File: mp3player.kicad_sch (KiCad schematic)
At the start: 6 parts, among them J1 AudioJack3, U1 ES8388, U2 ESP32-S3-WROOM-1

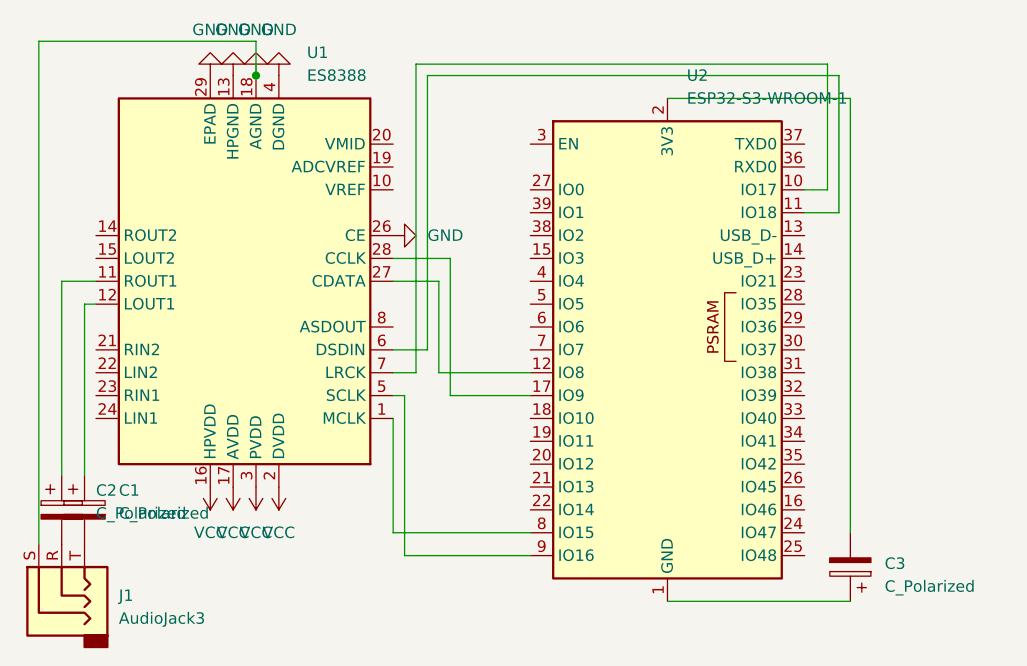
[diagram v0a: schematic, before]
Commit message: Autosave
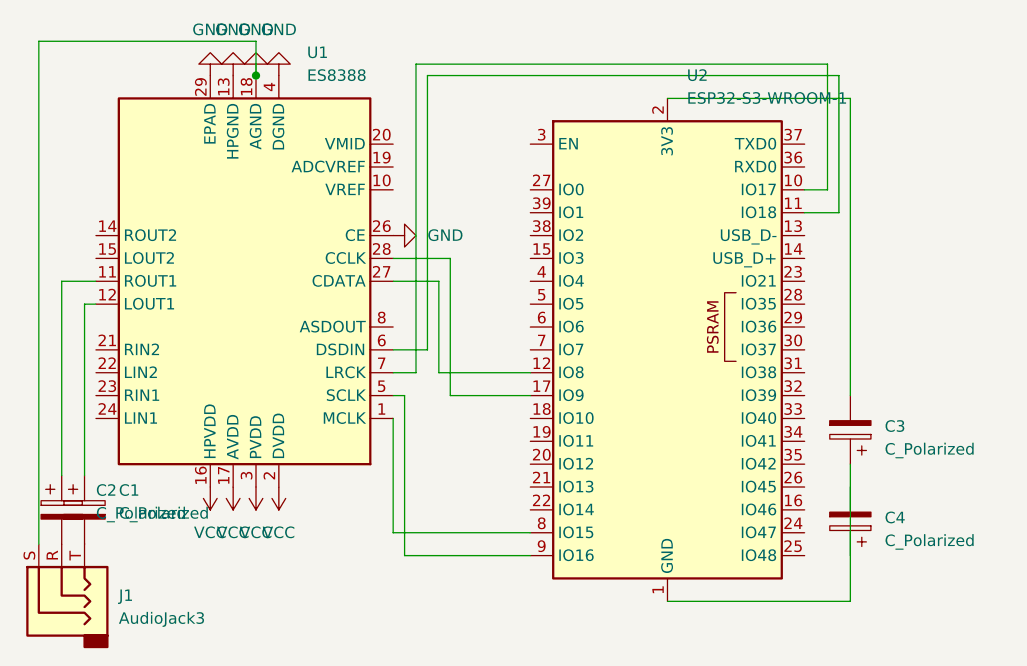
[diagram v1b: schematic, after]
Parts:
- added C4: C_Polarized, symbol Device:C_Polarized
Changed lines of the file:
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@@
 	(wire
 		(pts
-			(xy 105.41 19.05) (xy 105.41 67.31)
+			(xy 105.41 19.05) (xy 105.41 52.07)
 		)
 		(stroke
@@
 	(wire
 		(pts
-			(xy 21.59 41.91) (xy 20.32 41.91)
+			(xy 105.41 59.69) (xy 105.41 74.93)
 		)
 		(stroke
@@
 	(wire
 		(pts
-			(xy 59.69 49.53) (xy 69.85 49.53)
+			(xy 21.59 41.91) (xy 20.32 41.91)
 		)
 		(stroke
@@
 	(wire
 		(pts
-			(xy 58.42 46.99) (xy 54.61 46.99)
+			(xy 59.69 49.53) (xy 69.85 49.53)
 		)
 		(stroke
@@
 	(wire
 		(pts
-			(xy 58.42 16.51) (xy 58.42 46.99)
+			(xy 58.42 46.99) (xy 54.61 46.99)
 		)
 		(stroke
@@
 		)
 	)
+	(wire
+		(pts
+			(xy 58.42 16.51) (xy 58.42 46.99)
+		)
+		(stroke
+			(width 0)
+			(type default)
+		)
+	)
 	(symbol
 		(lib_id "power:VCC")
@@
 	)
 	(symbol
+		(lib_id "Device:C_Polarized")
+		(at 105.41 66.04 180)
+		(unit 1)
+		(body_style 1)
+		(exclude_from_sim no)
+		(in_bom yes)
+		(on_board yes)
+		(in_pos_files yes)
+		(dnp no)
+		(fields_autoplaced yes)
+		(property "Reference" "C4"
+			(at 109.22 65.6589 0)
+			(show_name no)
+			(do_not_autoplace no)
+			(effects
+				(font
+					(size 1.27 1.27)
+				)
+				(justify right)
+			)
+		)
+		(property "Value" "C_Polarized"
+			(at 109.22 68.1989 0)
+			(show_name no)
+			(do_not_autoplace no)
+			(effects
+				(font
+					(size 1.27 1.27)
+				)
+				(justify right)
+			)
+		)
+		(property "Footprint" ""
+			(at 104.4448 62.23 0)
+			(hide yes)
+			(show_name no)
+			(do_not_autoplace no)
+			(effects
+				(font
+					(size 1.27 1.27)
+				)
+			)
+		)
+		(property "Datasheet" ""
+			(at 105.41 66.04 0)
+			(hide yes)
+			(show_name no)
+			(do_not_autoplace no)
+			(effects
+				(font
+					(size 1.27 1.27)
+				)
+			)
+		)
+		(property "Description" "Polarized capacitor"
+			(at 105.41 66.04 0)
+			(hide yes)
+			(show_name no)
+			(do_not_autoplace no)
+			(effects
+				(font
+					(size 1.27 1.27)
+				)
+			)
+		)
+		(pin "1"
+		)
+		(pin "2"
+		)
+		(instances
+			(project "mp3player"
+				(path "/7851373b-cb7e-4e42-801a-d8b5ac5735f4"
+					(reference "C4")
+					(unit 1)
+				)
+			)
+		)
+	)
+	(symbol
+		(lib_id "Device:C_Polarized")
+		(at 105.41 55.88 180)
+		(unit 1)
+		(body_style 1)
+		(exclude_from_sim no)
+		(in_bom yes)
+		(on_board yes)
+		(in_pos_files yes)
+		(dnp no)
+		(fields_autoplaced yes)
+		(property "Reference" "C3"
+			(at 109.22 55.4989 0)
+			(show_name no)
+			(do_not_autoplace no)
+			(effects
+				(font
+					(size 1.27 1.27)
+				)
+				(justify right)
+			)
+		)
+		(property "Value" "C_Polarized"
+			(at 109.22 58.0389 0)
+			(show_name no)
+			(do_not_autoplace no)
+			(effects
+				(font
+					(size 1.27 1.27)
+				)
+				(justify right)
+			)
+		)
+		(property "Footprint" ""
+			(at 104.4448 52.07 0)
+			(hide yes)
+			(show_name no)
+			(do_not_autoplace no)
+			(effects
+				(font
+					(size 1.27 1.27)
+				)
+			)
+		)
+		(property "Datasheet" ""
+			(at 105.41 55.88 0)
+			(hide yes)
+			(show_name no)
+			(do_not_autoplace no)
+			(effects
+				(font
+					(size 1.27 1.27)
+				)
+			)
+		)
+		(property "Description" "Polarized capacitor"
+			(at 105.41 55.88 0)
+			(hide yes)
+			(show_name no)
+			(do_not_autoplace no)
+			(effects
+				(font
+					(size 1.27 1.27)
+				)
+			)
+		)
+		(pin "1"
+		)
+		(pin "2"
+		)
+		(instances
+			(project "mp3player"
+				(path "/7851373b-cb7e-4e42-801a-d8b5ac5735f4"
+					(reference "C3")
+					(unit 1)
+				)
+			)
+		)
+	)
+	(symbol
 		(lib_id "Connector_Audio:AudioJack3")
 		(at 17.78 73.66 90)
@@
 					(unit 1)
 				)
-			)
-		)
-	)
-	(symbol
-		(lib_id "Device:C_Polarized")
-		(at 105.41 71.12 180)
-		(unit 1)
-		(body_style 1)
-		(exclude_from_sim no)
-		(in_bom yes)
-		(on_board yes)
-		(in_pos_files yes)
-		(dnp no)
-		(fields_autoplaced yes)
-		(property "Reference" "C3"
-			(at 109.22 70.7389 0)
-			(show_name no)
-			(do_not_autoplace no)
-			(effects
-				(font
-					(size 1.27 1.27)
-				)
-				(justify right)
-			)
-		)
-		(property "Value" "C_Polarized"
-			(at 109.22 73.2789 0)
-			(show_name no)
-			(do_not_autoplace no)
-			(effects
-				(font
-					(size 1.27 1.27)
-				)
-				(justify right)
-			)
-		)
-		(property "Footprint" ""
-			(at 104.4448 67.31 0)
-			(hide yes)
-			(show_name no)
-			(do_not_autoplace no)
-			(effects
-				(font
-					(size 1.27 1.27)
-				)
-			)
-		)
-		(property "Datasheet" ""
-			(at 105.41 71.12 0)
-			(hide yes)
-			(show_name no)
-			(do_not_autoplace no)
-			(effects
-				(font
-					(size 1.27 1.27)
-				)
-			)
-		)
-		(property "Description" "Polarized capacitor"
-			(at 105.41 71.12 0)
-			(hide yes)
-			(show_name no)
-			(do_not_autoplace no)
-			(effects
-				(font
-					(size 1.27 1.27)
-				)
-			)
-		)
-		(pin "1"
-		)
-		(pin "2"
-		)
-		(instances
-			(project "mp3player"
-				(path "/7851373b-cb7e-4e42-801a-d8b5ac5735f4"
-					(reference "C3")
-					(unit 1)
-				)

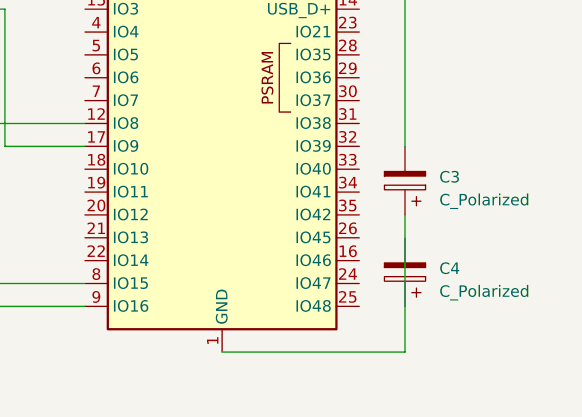
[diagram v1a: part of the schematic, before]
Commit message: Autosave
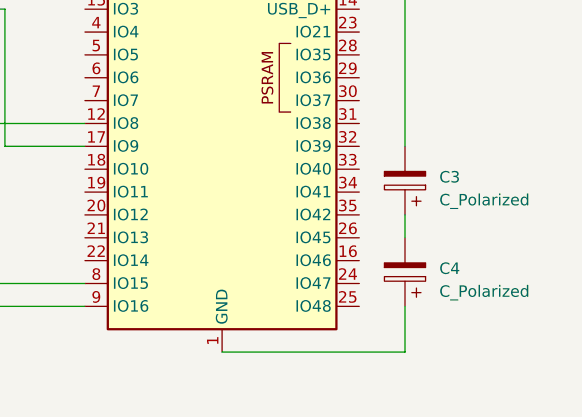
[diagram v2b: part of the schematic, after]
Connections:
- net at C4.1: now also U2.1 (GND), U2.40 (GND), U2.41 (GND)
- net at C4.2: now also C3.1
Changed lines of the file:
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@@
+	(wire
+		(pts
+			(xy 105.41 69.85) (xy 105.41 74.93)
+		)
+		(stroke
+			(width 0)
+			(type default)
+		)
+	)
 	(wire
 		(pts
@@
 	(wire
 		(pts
-			(xy 105.41 59.69) (xy 105.41 74.93)
+			(xy 105.41 59.69) (xy 105.41 62.23)
 		)
 		(stroke
